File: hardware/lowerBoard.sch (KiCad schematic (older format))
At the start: 21 parts, among them J10 Screw_Terminal_01x02, J11 Screw_Terminal_01x02, J12 Screw_Terminal_01x02, J13 Screw_Terminal_01x02, J14 Screw_Terminal_01x02, J15 Screw_Terminal_01x02, J16 Screw_Terminal_01x02, J17 Screw_Terminal_01x02, J18 Screw_Terminal_01x02, J19 Screw_Terminal_01x02, J20 Screw_Terminal_01x02, J3 Screw_Terminal_01x02, J4 Screw_Terminal_01x02, J5 Screw_Terminal_01x02, J6 Screw_Terminal_01x02, J7 Screw_Terminal_01x02, J8 Screw_Terminal_01x02, J9 Conn_02x10_Odd_Even, U5 R-783.3-0.5

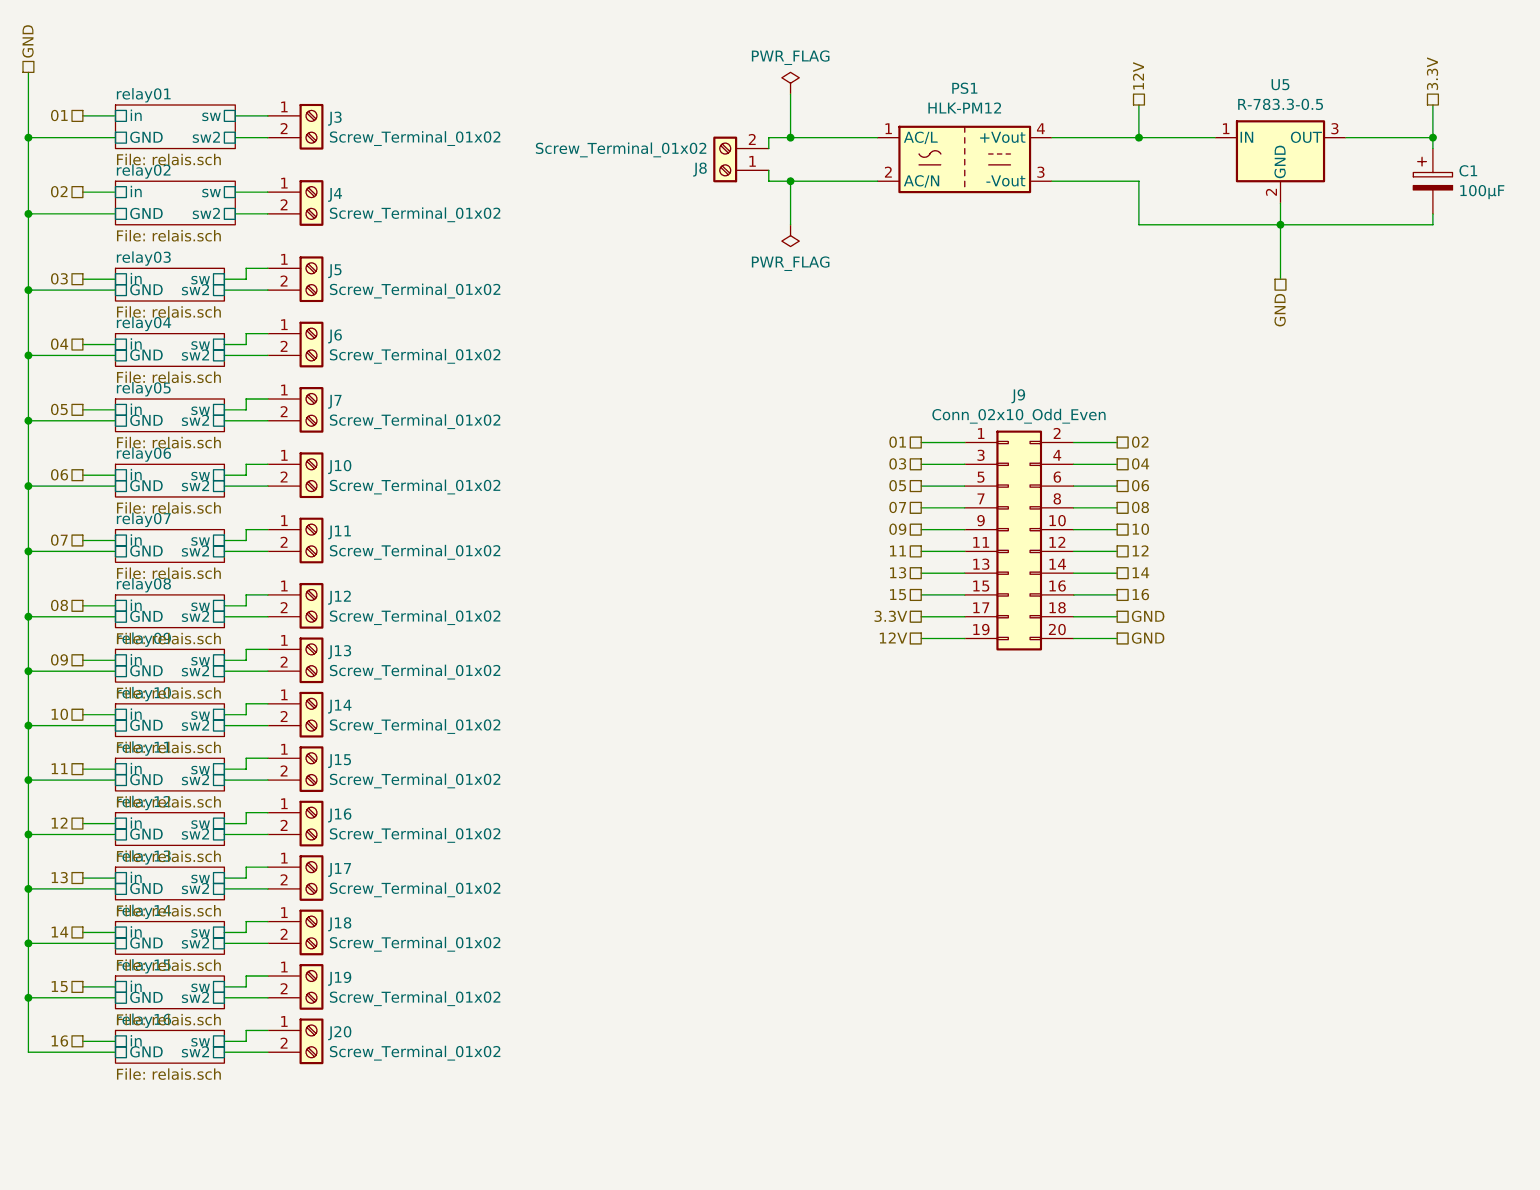
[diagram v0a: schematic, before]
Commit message: continue to design lower pcb
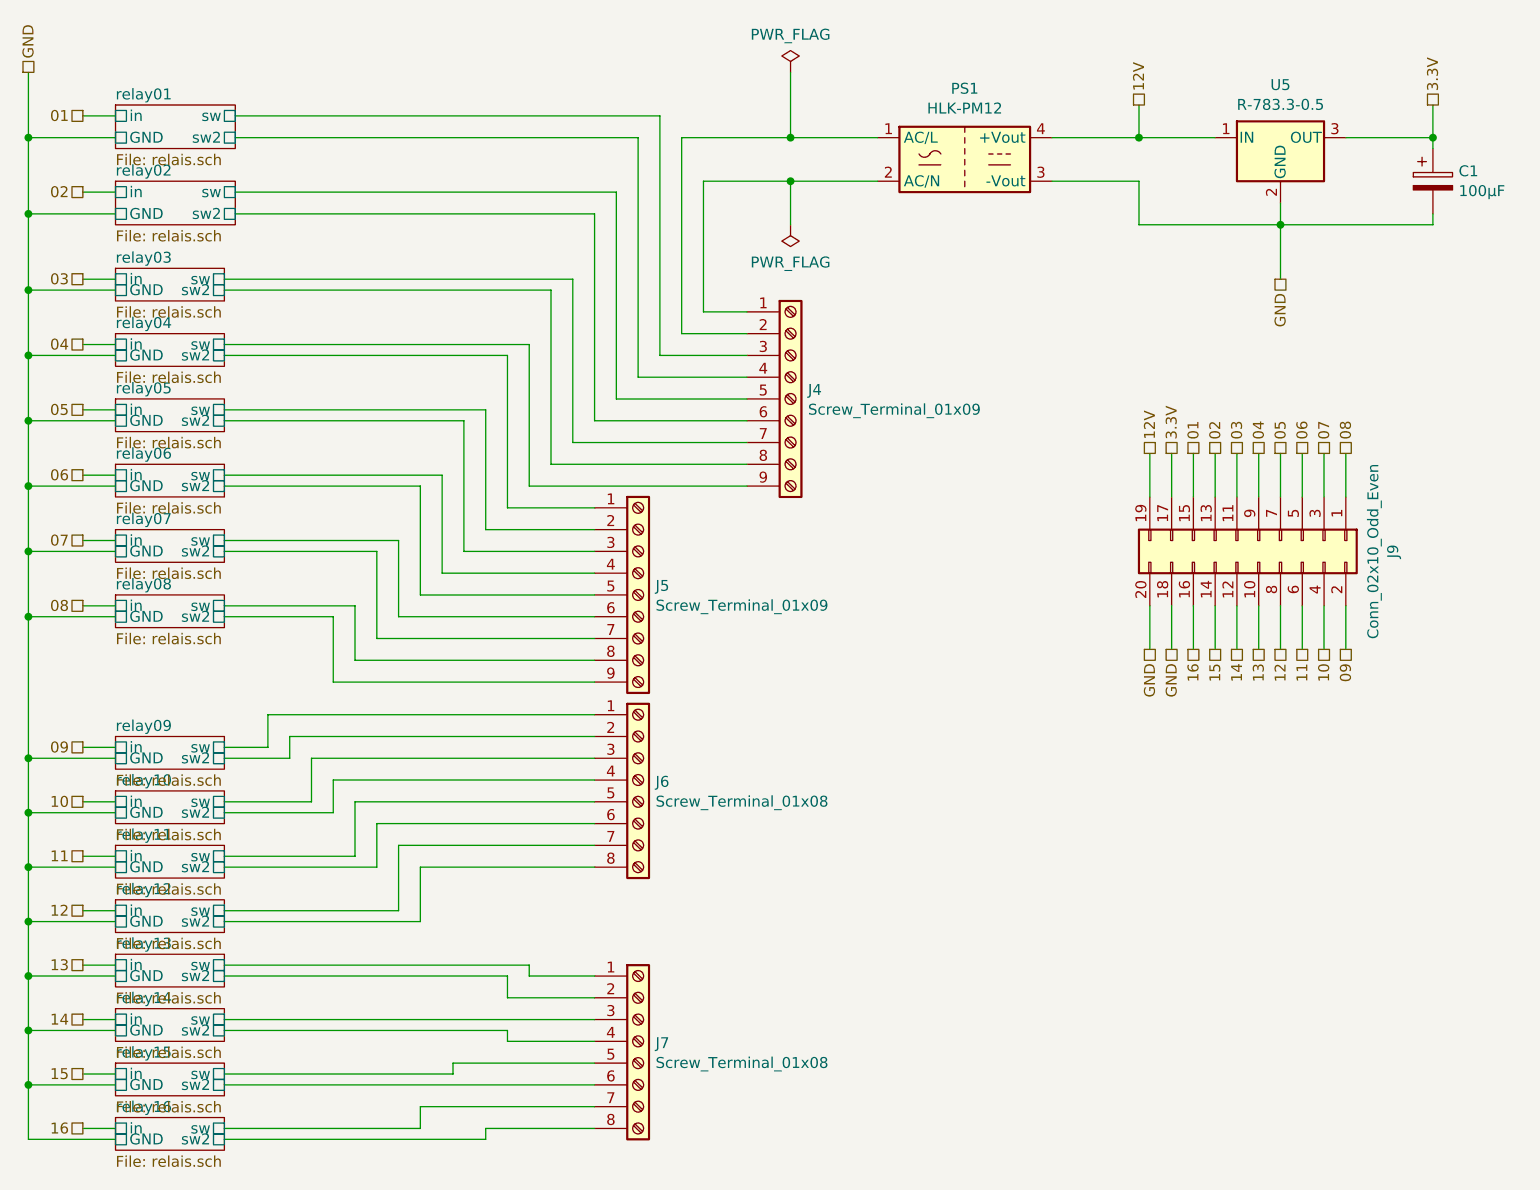
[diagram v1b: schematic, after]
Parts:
- removed J10, J11, J12, J13, J14, J15, J16, J17, J18, J19, J20, J3, J4, J5, J6, J7, J8: Screw_Terminal_01x02, TerminalBlock_MetzConnect:TerminalBlock_MetzConnect_Type059_RT06302HBWC_1x02_P3.50mm_Horizontal, symbol Connector:Screw_Terminal_01x02
- added J4, J5: Screw_Terminal_01x09, TerminalBlock_RND:TerminalBlock_RND_205-00239_1x09_P5.08mm_Horizontal, symbol Connector:Screw_Terminal_01x09
- added J6, J7: Screw_Terminal_01x08, TerminalBlock_RND:TerminalBlock_RND_205-00238_1x08_P5.08mm_Horizontal, symbol Connector:Screw_Terminal_01x08
- renumbered J9 to J3
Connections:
- net 01: now also J3.15 (Pin_15); no longer J3.1 (Pin_1)
- net 02: now also J3.13 (Pin_13); no longer J3.2 (Pin_2)
- net 03: now also J3.11 (Pin_11); no longer J3.3 (Pin_3)
- net 04: now also J3.9 (Pin_9); no longer J3.4 (Pin_4)
- net 05: now also J3.7 (Pin_7); no longer J3.5 (Pin_5)
- net 06: now also J3.5 (Pin_5); no longer J3.6 (Pin_6)
- net 07: now also J3.3 (Pin_3); no longer J3.7 (Pin_7)
- net 08: now also J3.1 (Pin_1); no longer J3.8 (Pin_8)
- net 09: now also J3.2 (Pin_2); no longer J3.9 (Pin_9)
- net 10: now also J3.4 (Pin_4); no longer J3.10 (Pin_10)
- net 11: now also J3.6 (Pin_6); no longer J3.11 (Pin_11)
- net 12: now also J3.8 (Pin_8); no longer J3.12 (Pin_12)
- net 13: now also J3.10 (Pin_10); no longer J3.13 (Pin_13)
- net 14: now also J3.12 (Pin_12); no longer J3.14 (Pin_14)
- net 15: now also J3.14 (Pin_14); no longer J3.15 (Pin_15)
- net relay01/sw: now also J4.3 (Pin_3)
- net relay01/sw2: now also J4.4 (Pin_4)
- net relay02/sw: now also J4.5 (Pin_5)
- net relay02/sw2: now also J4.6 (Pin_6)
- net relay03/sw: now also J4.7 (Pin_7)
- net relay03/sw2: now also J4.8 (Pin_8)
- net relay04/sw: now also J4.9 (Pin_9)
- net relay04/sw2: now also J5.1 (Pin_1)
- net relay05/sw: now also J5.2 (Pin_2)
- net relay05/sw2: now also J5.3 (Pin_3)
- net relay06/sw: now also J5.4 (Pin_4)
- net relay06/sw2: now also J5.5 (Pin_5)
- net relay07/sw: now also J5.6 (Pin_6)
- net relay07/sw2: now also J5.7 (Pin_7)
- net relay08/sw: now also J5.8 (Pin_8)
- net relay08/sw2: now also J5.9 (Pin_9)
- net relay09/sw: now also J6.1 (Pin_1)
- net relay09/sw2: now also J6.2 (Pin_2)
- net relay10/sw: now also J6.3 (Pin_3)
- net relay10/sw2: now also J6.4 (Pin_4)
- net relay11/sw: now also J6.5 (Pin_5)
- net relay11/sw2: now also J6.6 (Pin_6)
- net relay12/sw: now also J6.7 (Pin_7)
- net relay12/sw2: now also J6.8 (Pin_8)
- net relay13/sw: now also J7.1 (Pin_1)
- net relay13/sw2: now also J7.2 (Pin_2)
- net relay14/sw: now also J7.3 (Pin_3)
- net relay14/sw2: now also J7.4 (Pin_4)
- net relay15/sw: now also J7.5 (Pin_5)
- net relay15/sw2: now also J7.6 (Pin_6)
- net relay16/sw: now also J7.7 (Pin_7)
- net relay16/sw2: now also J7.8 (Pin_8)
- net at PS1.1 (AC/L): now also J4.2 (Pin_2)
- net at PS1.2 (AC/N): now also J4.1 (Pin_1)
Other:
- moved on the sheet: J9
